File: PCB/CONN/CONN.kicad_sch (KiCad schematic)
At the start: 25 parts, among them J1 Conn_02x06_Odd_Even, J2 Solar cell, J3 Conn_02x06_Odd_Even, J4 BM06B-SRSS-TBT(LF)(SN), J5 BM06B-SRSS-TBT(LF)(SN), J6 BM06B-SRSS-TBT(LF)(SN), J7 BM06B-SRSS-TBT(LF)(SN), J8 BM06B-SRSS-TBT(LF)(SN), J9 BM06B-SRSS-TBT(LF)(SN), U1 TCA9548APWR

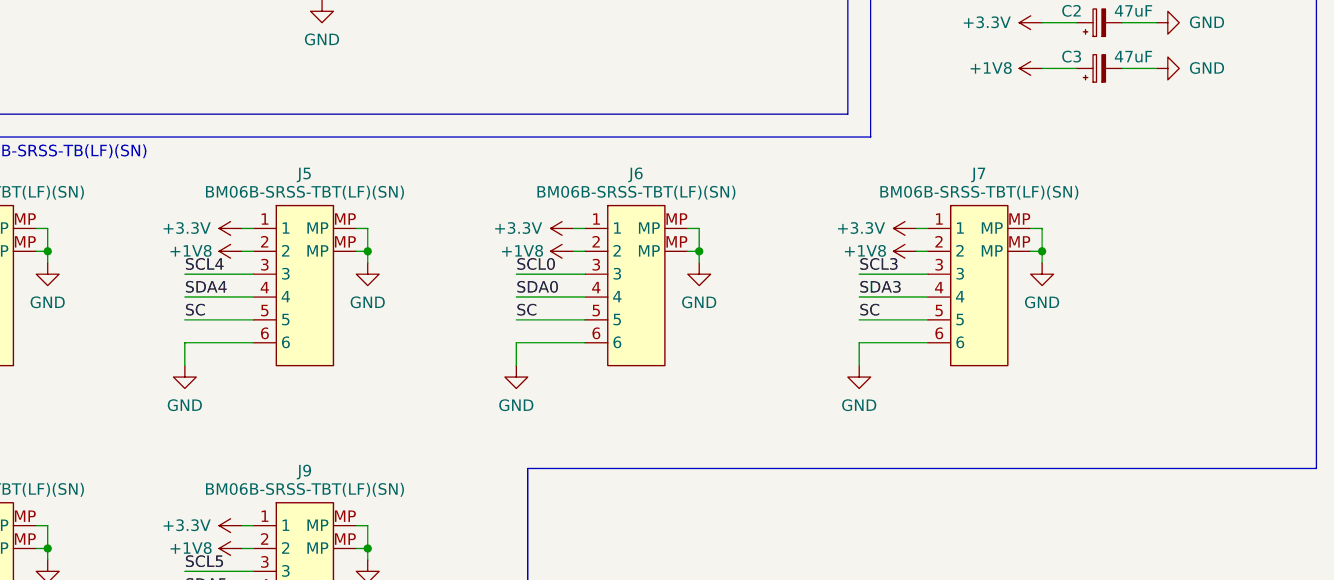
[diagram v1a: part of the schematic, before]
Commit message: udated by FZ from Windows
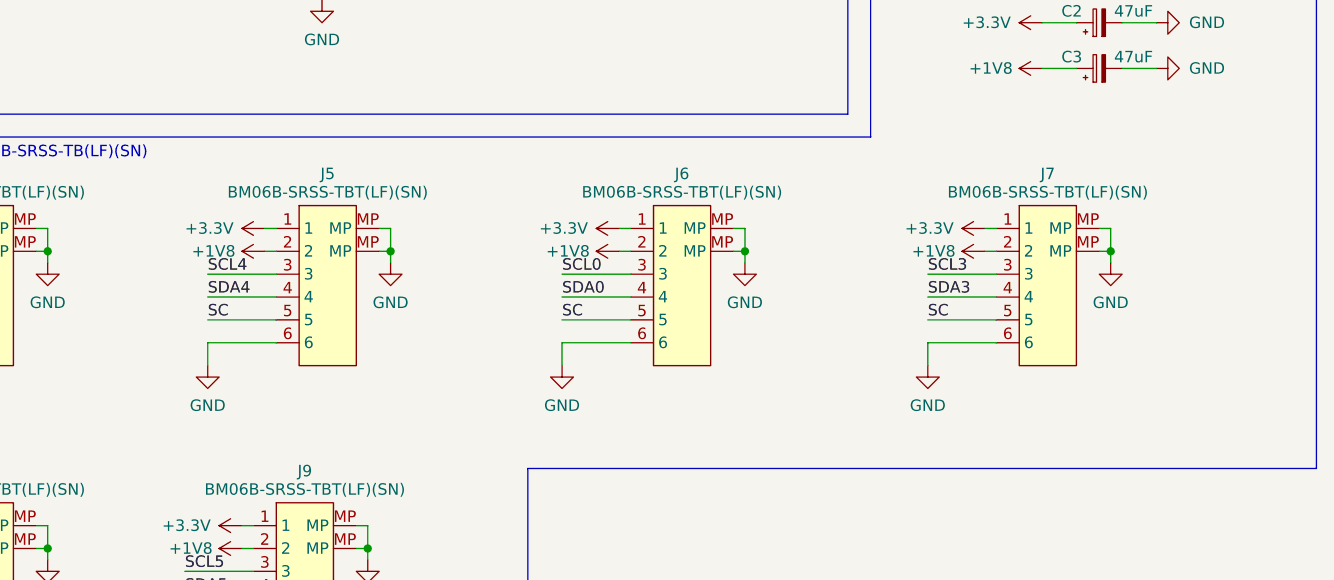
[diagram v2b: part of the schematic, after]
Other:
- moved on the sheet: J5, J6, J7
